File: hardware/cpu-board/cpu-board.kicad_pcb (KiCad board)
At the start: 2 copper layers, 160 x 100 mm, 46 parts, among them CON1 BARREL_JACK, P1 CTRL1, P2 CTRL2, P3 DATA, P4 IO, P5 ADDR1, P6 ADDR2, P7 SERIAL, SW1 RESET, SW2 PWR, U1 WD65C02, U10 W65C51N, U2 AT28C256, U3 74HC132, U4 CY7C199, U5 MXO45HS, U6 7805, U7 4012, U8 4012, U9 74HC138, X1 CRYSTAL

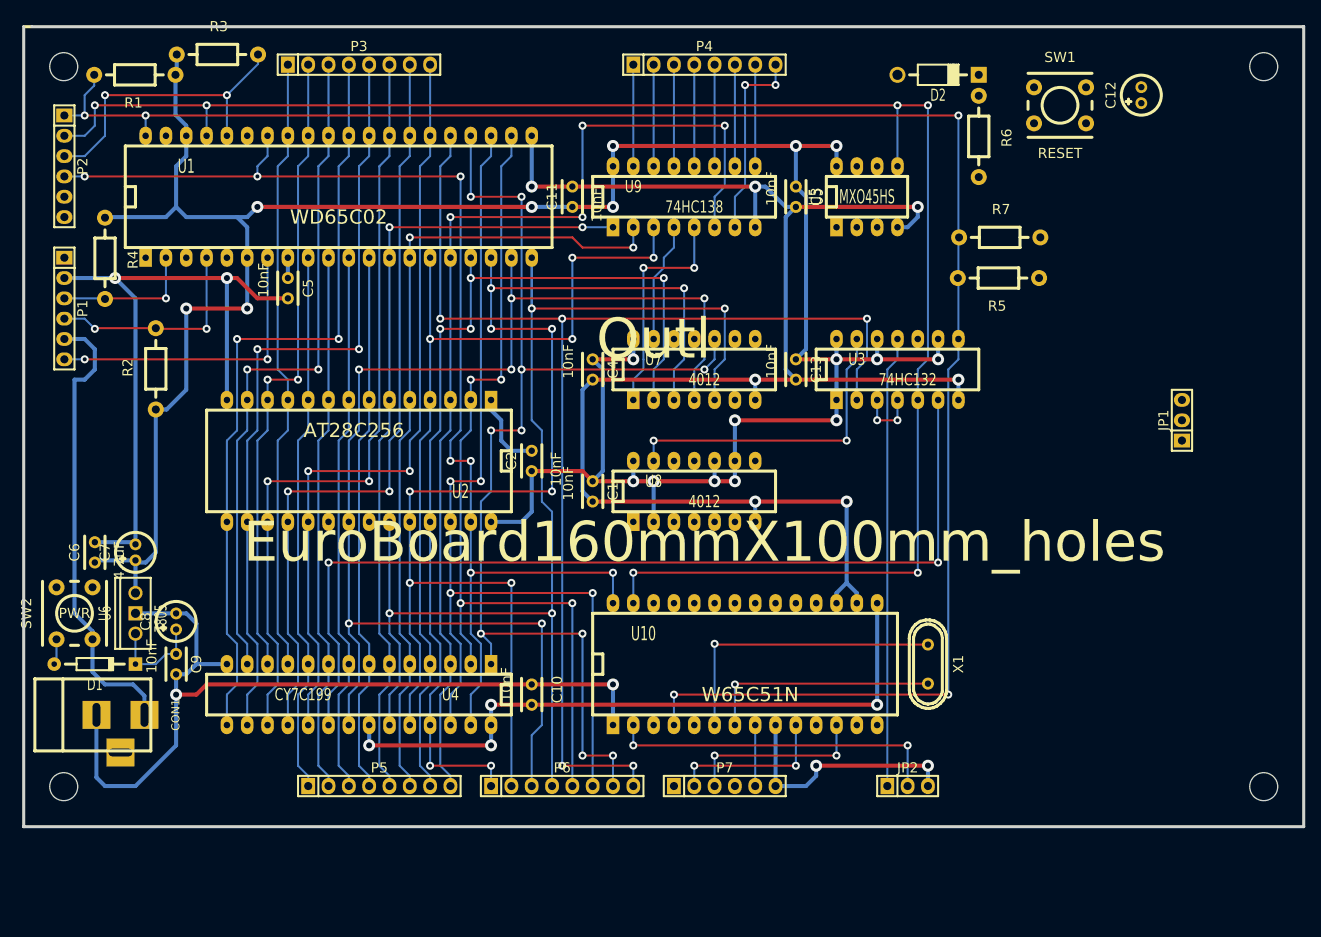
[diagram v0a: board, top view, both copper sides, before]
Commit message: finish layout
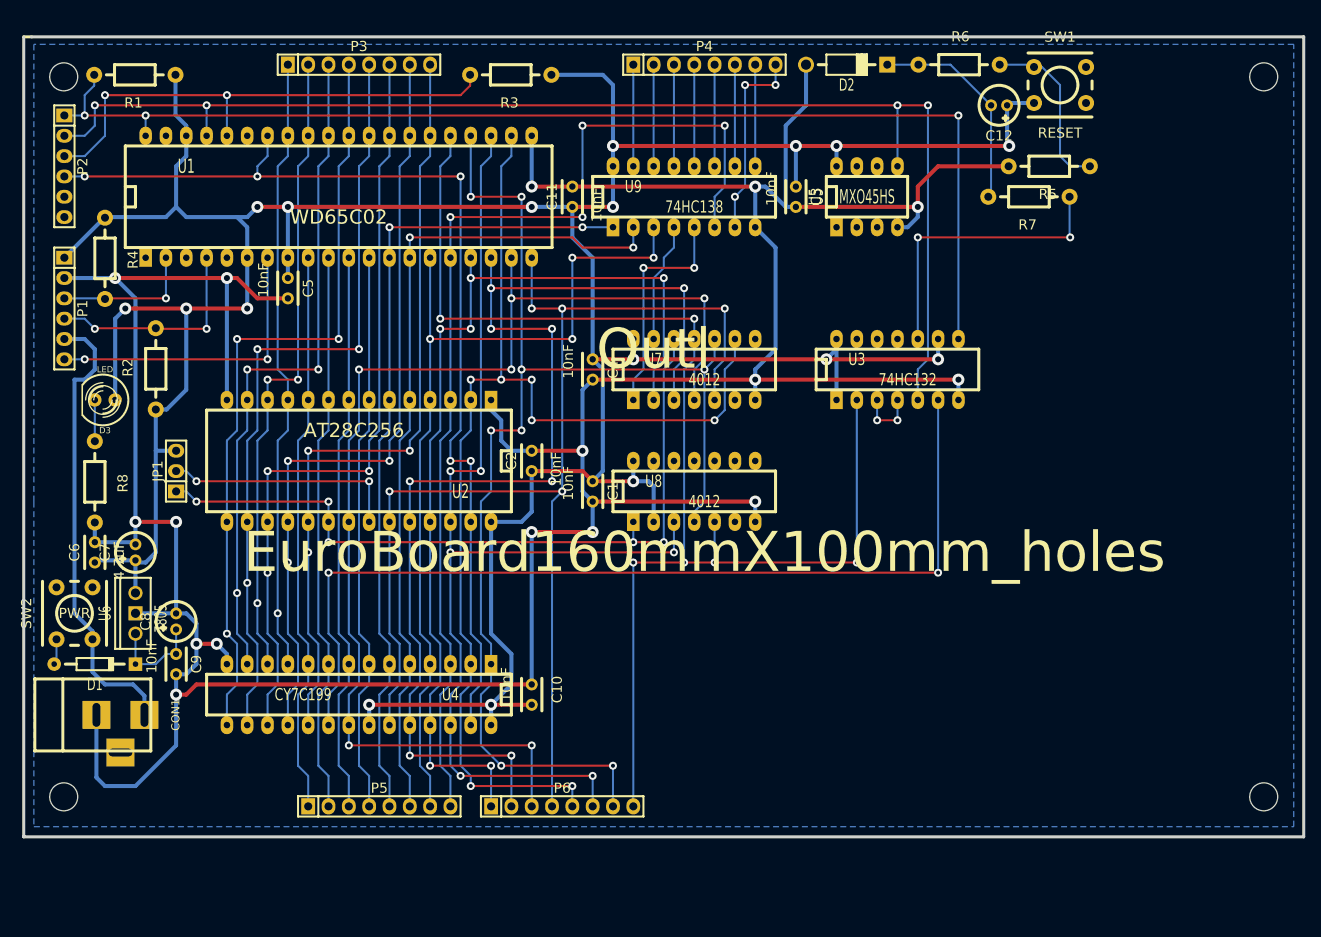
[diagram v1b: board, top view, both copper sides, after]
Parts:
- removed C13: 10nF, Capacitors_ThroughHole:Capacitor4x3RM2.5
- removed JP2: JUMPER3, Pin_Headers:Pin_Header_Straight_1x03
- removed P7: SERIAL, Socket_Strips:Socket_Strip_Straight_1x06
- removed U10: W65C51N, Sockets_DIP:DIP-28__600_ELL
- removed X1: CRYSTAL, Crystals:Crystal_HC49-U_Vertical
- added D3: LED, LEDs:LED-5MM, F.Cu at (44.5, 82.5)
- added R8: 330, Resistors_ThroughHole:Resistor_Horizontal_RM10mm, F.Cu at (43.2, 92.7)
- moved JP1 125.9 mm to (53.3, 91.4)
- moved R3 36.9 mm to (95.2, 41.9), turned to 180 degrees
- moved C12 17.8 mm to (156.2, 45.7), turned to 180 degrees
- moved R5 15.3 mm to (162.6, 53.3)
- moved D2 11.5 mm to (137.2, 40.6)
- moved R6 9.25 mm to (151.1, 40.6), turned to 0 degrees
- moved R7 6.35 mm to (160.0, 57.1), turned to 180 degrees
- moved SW1 2.54 mm to (163.8, 43.2)
- moved P5 2.54 mm to (78.7, 133.3)
- moved P6 2.54 mm to (101.6, 133.3)
- moved Outl 1.27 mm to (34.3, 137.2)
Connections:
- U3 pad 11: /IO/ACAISEL -> (no net)
- U3 pad 12: +5V -> (no net)
- U3 pad 13: Net-(U3-Pad13) -> (no net)
- U8 pad 10: +5V -> (no net)
- U8 pad 11: A2 -> (no net)
- U8 pad 12: A3 -> (no net)
- U8 pad 13: Net-(U3-Pad13) -> (no net)
- U8 pad 9: +5V -> (no net)
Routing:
- net /Address Decode/~ROMSEL: track 0.00 -> 95.0 mm, vias 0 -> 5
- net ~RST: track 230.9 -> 147.8 mm, vias 5 -> 3
- net PHI2: track 220.8 -> 159.8 mm, vias 6 -> 4
- net /IO/ACAISEL: track 56.4 -> 0.00 mm
- net /IO/ACAIEN: track 41.9 -> 0.00 mm, vias 2 -> 0
- net Net-(U3-Pad13): track 39.9 -> 0.00 mm, vias 2 -> 0
- net A12: track 108.3 -> 145.9 mm, vias 4 -> 7
- net /IO/XTLI: track 36.9 -> 0.00 mm, vias 1 -> 0
- net Net-(R7-Pad1): track 0.00 -> 36.9 mm, vias 0 -> 2
- net /~ROMOE: track 0.00 -> 29.7 mm, vias 0 -> 2
- net /IO/XTLO: track 29.3 -> 0.00 mm, vias 1 -> 0
- net +5V: track 426.4 -> 454.7 mm, vias 22 -> 17
- net Net-(C12-Pad2): track 0.00 -> 26.6 mm
- net BE: track 38.2 -> 63.8 mm
- net /IO/RX: track 22.9 -> 0.00 mm, vias 2 -> 0
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- added copper zone on B.Cu, net GND

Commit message: first pcb layout
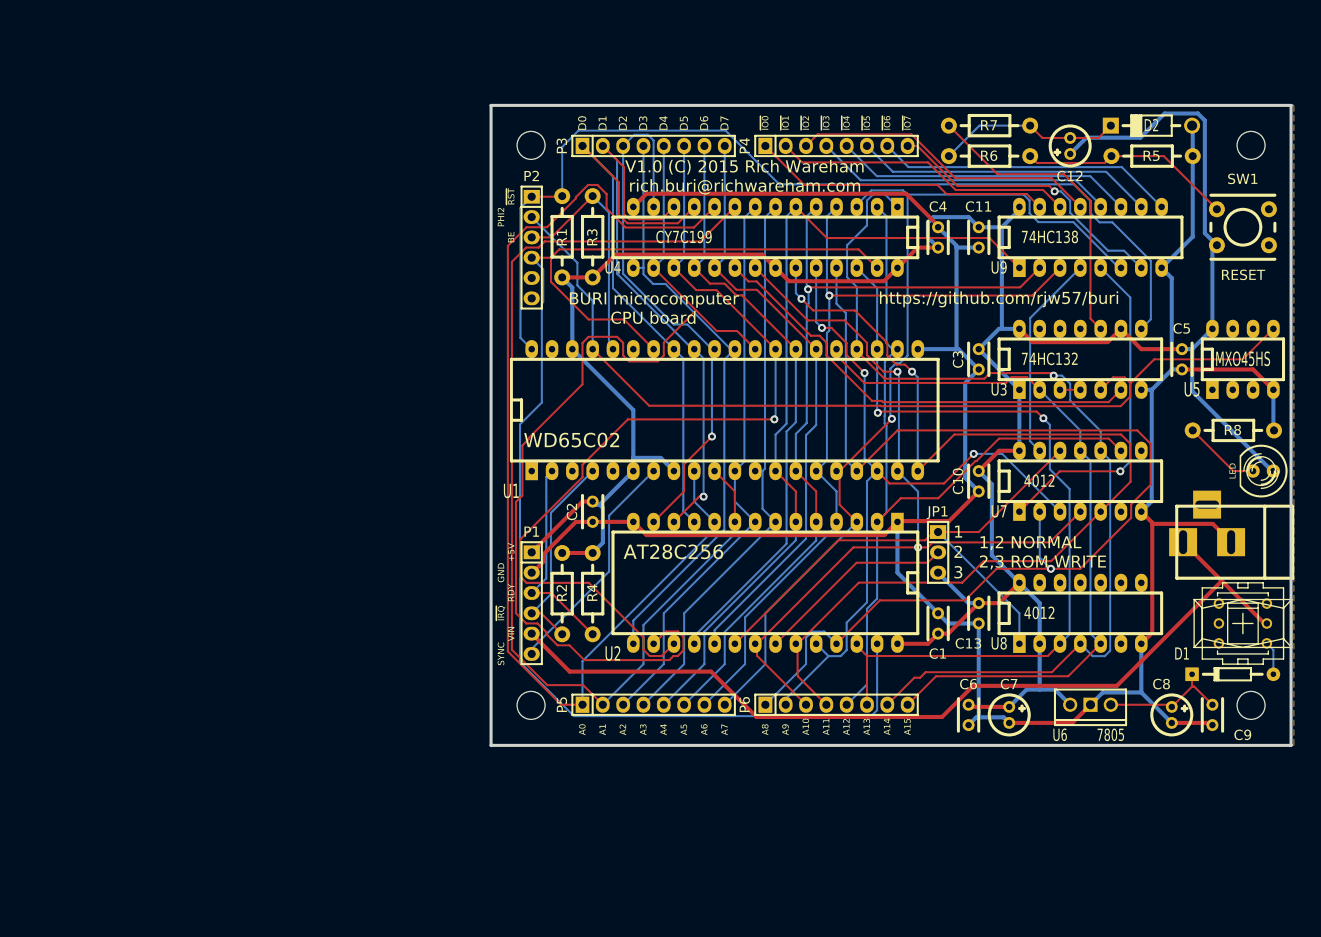
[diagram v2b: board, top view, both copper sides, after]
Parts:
- removed the Outl at (34.3, 137.2)
- removed SW2: PWR, IHeartKiCad:SW_M6_PTH
- added C13: 10nF, Capacitors_ThroughHole:Capacitor4x3RM2.5, F.Cu at (153.7, 108.0)
- added Outl: EuroBoard_halb_Type-I_100mmX80mm_holes, EuroBoard_Outline:EuroBoard_halb_Type-I_100mmX80mm_holes, F.Cu at (92.7, 125.7)
- added S1: PWR, switch-misc-PVA2F, F.Cu at (186.7, 110.5)
- moved D3 145.1 mm to (189.2, 91.4)
- moved CON1 143.9 mm to (185.4, 100.3), turned to 180 degrees
- moved R8 142.4 mm to (185.4, 86.4), turned to 0 degrees
- moved D1 142.2 mm to (185.4, 116.8), turned to 180 degrees
- moved C9 129.7 mm to (182.9, 120.7)
- moved C8 125.0 mm to (177.8, 121.9), turned to 270 degrees
- moved U6 119.9 mm to (167.6, 120.7), turned to 270 degrees
- moved C5 112.1 mm to (179.1, 76.2)
- moved C7 111.1 mm to (157.5, 121.9), turned to 270 degrees
- moved C6 110.7 mm to (152.4, 120.7), turned to 270 degrees
- moved JP1 95.8 mm to (148.6, 101.6), turned to 270 degrees
- moved U4 76.5 mm to (127.0, 62.2)
- moved R4 74.0 mm to (105.4, 106.7)
- moved P1 69.1 mm to (97.8, 108.0)
- moved C10 63.1 mm to (153.7, 91.4), turned to 270 degrees
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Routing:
- net GND: track 455.6 -> 318.9 mm, vias 16 -> 0
- net +5V: track 454.7 -> 333.0 mm, vias 17 -> 0
- net A15: track 170.0 -> 90.7 mm, vias 6 -> 0
- net A0: track 70.7 -> 133.3 mm
- net /~RAMCE: track 117.9 -> 56.8 mm, vias 2 -> 0
- net A1: track 70.7 -> 130.5 mm
- net VIN: track 57.5 -> 112.3 mm
- net A9: track 146.4 -> 94.3 mm, vias 8 -> 3
- net A10: track 149.4 -> 104.9 mm, vias 6 -> 2
- net R/~W: track 127.8 -> 172.3 mm, vias 5 -> 0
- net A12: track 145.9 -> 101.6 mm, vias 7 -> 0
- net PHI2: track 159.8 -> 117.4 mm, vias 4 -> 0
- net A14: track 157.4 -> 121.4 mm, vias 8 -> 1
- net A13: track 138.0 -> 103.3 mm, vias 6 -> 2
- net BE: track 63.8 -> 29.9 mm, vias 2 -> 0
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- added copper zone on F.Cu, net GND
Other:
- board size 160 x 100 mm -> 100 x 80 mm
- rule via_min_drill: 0.8 -> 0.5
- rule via_min_size: 1 -> 0.8
- board text added: "+5V"
- board text added: "1"
- board text added: "1,2 NORMAL 2,3 ROM WRITE"
- board text added: "2"
- board text added: "3"
- board text added: "A0"
- board text added: "A1"
- board text added: "A10"
- board text added: "A11"
- board text added: "A12"
- board text added: "A13"
- board text added: "A14"
- board text added: "A15"
- board text added: "A2"
- board text added: "A3"
- board text added: "A4"
- board text added: "A5"
- board text added: "A6"
- board text added: "A7"
- board text added: "A8"
- board text added: "A9"
- board text added: "BE"
- board text added: "BURI microcomputer CPU board"
- board text added: "D0"
- board text added: "D1"
- board text added: "D2"
- board text added: "D3"
- board text added: "D4"
- board text added: "D5"
- board text added: "D6"
- board text added: "D7"
- board text added: "GND"
- board text added: "PHI2"
- board text added: "RDY"
- board text added: "SYNC"
- board text added: "V1.0 (C) 2015 Rich Wareham rich.buri@richwareham.com"
- board text added: "VIN"
- board text added: "https://github.com/rjw57/buri"
- board text added: "~IO0"
- board text added: "~IO1"
- board text added: "~IO2"
- board text added: "~IO3"
- board text added: "~IO4"
- board text added: "~IO5"
- board text added: "~IO6"
- board text added: "~IO7"
- board text added: "~IRQ"
- board text added: "~RST"

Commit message: final version sent to manufacturer
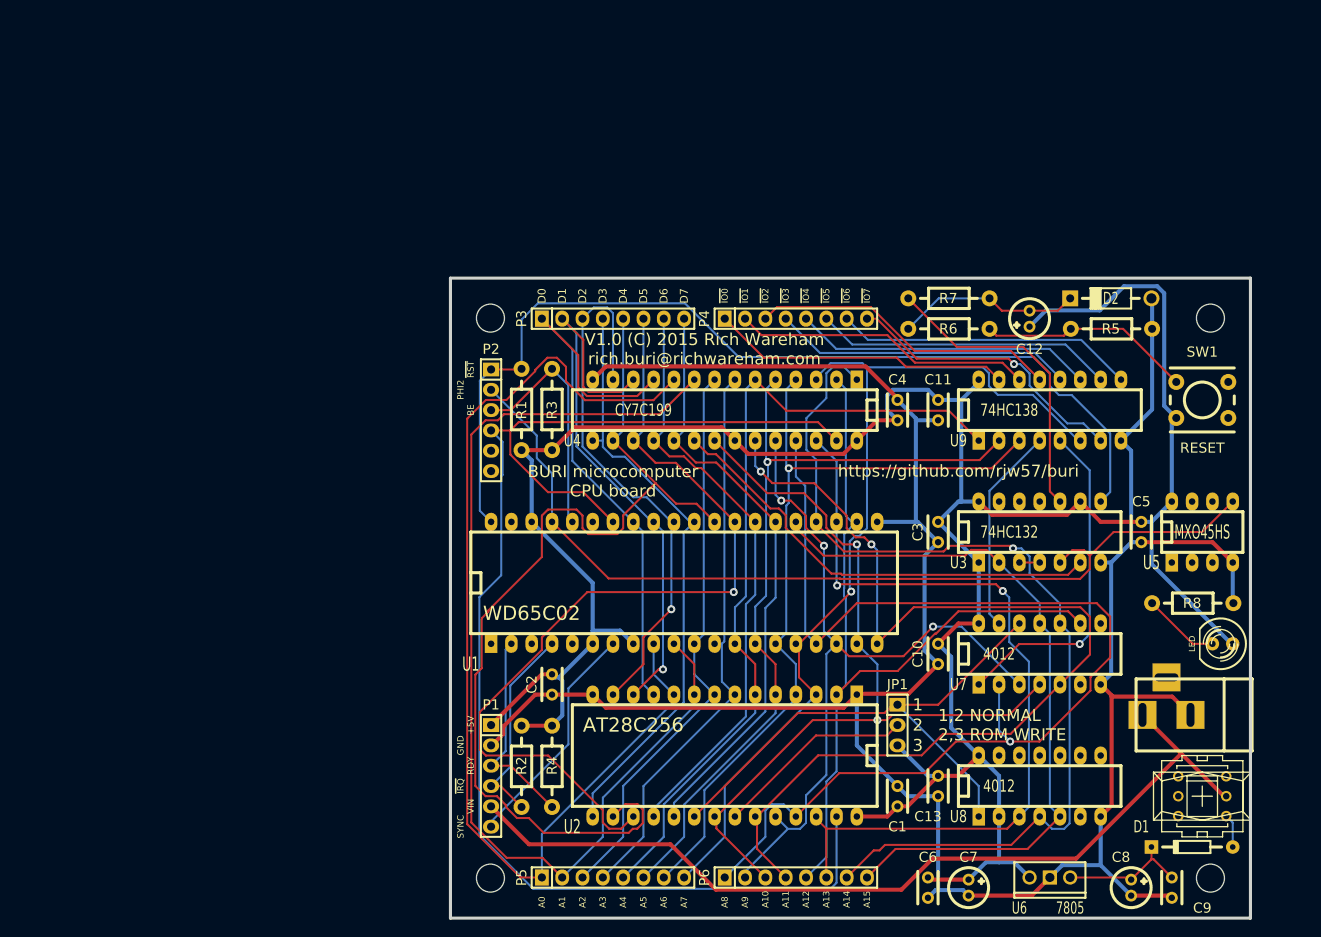
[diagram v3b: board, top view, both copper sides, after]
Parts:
- moved S1 22.2 mm to (181.6, 132.1)
- moved C4 22.2 mm to (143.5, 85.1)
- moved C6 22.2 mm to (147.3, 142.2)
- moved JP1 22.2 mm to (143.5, 123.2)
- moved P2 22.2 mm to (92.7, 85.1)
- moved U3 22.2 mm to (161.3, 99.1)
- moved U7 22.2 mm to (161.3, 114.3)
- moved U8 22.2 mm to (161.3, 130.8)
- moved C10 22.2 mm to (148.6, 113.0)
- moved C12 22.2 mm to (160.0, 72.4)
- moved C2 22.2 mm to (100.3, 116.8)
- moved C3 22.2 mm to (148.6, 97.8)
- moved C5 22.2 mm to (174.0, 97.8)
- moved C9 22.2 mm to (177.8, 142.2)
- moved CON1 22.2 mm to (180.3, 121.9)
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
